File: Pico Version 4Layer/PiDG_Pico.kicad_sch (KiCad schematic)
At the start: 83 parts, among them J1 Conn_02x05_Odd_Even, J10 Trig, J11 Laser Enable, J12 Pixel Reset, J14 Pico Socket A, J15 Pico Socket B, J16 Laser En/PWM Trig/GND, J17 USB-C PD in, J18 Laser 1 mode, J19 Laser 2 mode, J2 Conn_02x05_Odd_Even, J3 Conn_02x05_Odd_Even, J4 Conn_02x05_Odd_Even, J5 Conn_02x05_Odd_Even, J6 Conn_02x05_Odd_Even, J7 Laser 1, J8 Laser 2, U1 74LVC1G04, U10 74AHCT1G08, U11 Raspberry Pi Pico 2 W, U12 74LVC1G17, U13 UCC27524, U14 CH224K, U15 AP63205WU, U16 LM66100, U17 LT3065EDD, U18 TPS3700DDC, U2 SN74LVC04AD, U3 74LVC1G00, U4 SN74LVC04AD, U5 74LVC1G04, U6 SN74LVC04AD, U7 74AHCT1G08, U8 74AHCT1G08, U9 NCP718xSN180

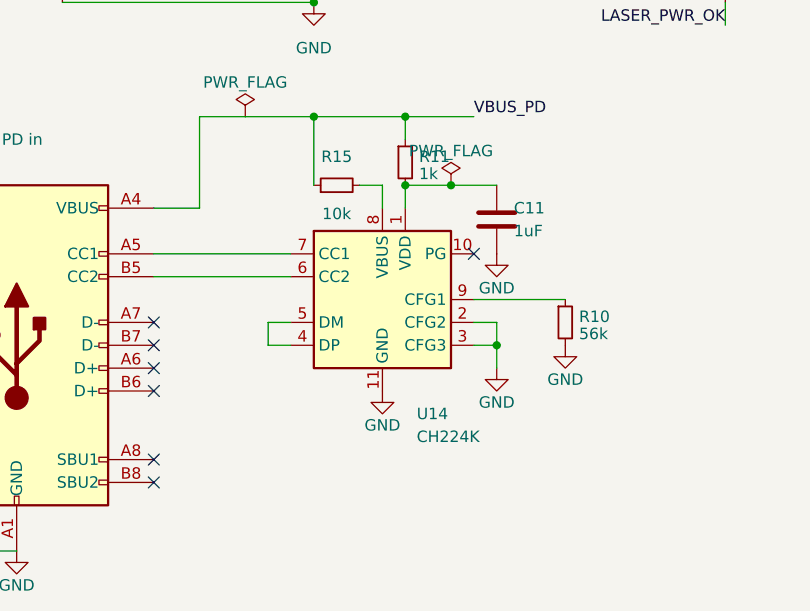
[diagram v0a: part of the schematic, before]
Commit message: Update Pico hardware and fabrication files
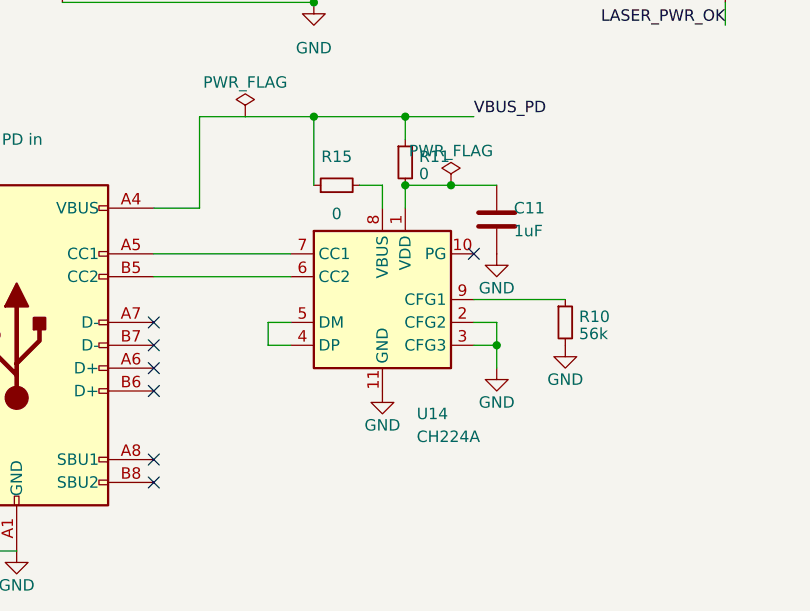
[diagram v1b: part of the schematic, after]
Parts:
- R11: value 1k -> 0
- R15: value 10k -> 0
- U14: value CH224K -> CH224A
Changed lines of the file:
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@@
 			)
 		)
-		(property "Value" "10k"
+		(property "Value" "0"
 			(at 360.68 155.575 90)
 			(show_name no)
@@
 			)
 		)
-		(property "Description" "CH224K VBUS sense resistor (datasheet: 10k)"
+		(property "Description" "CH224A VBUS (pin 8) shorted to VHV: 0 ohm, per WCH guide 7.2.1 (was 10k for CH224K)"
 			(at 360.68 152.4 0)
 			(hide yes)
@@
 			)
 		)
-		(property "Value" "CH224K"
+		(property "Value" "CH224A"
 			(at 369.57 180.34 0)
 			(show_name no)
@@
 			)
 		)
-		(property "Description" "USB PD sink controller. R10 = 56k on CFG1 requests 15 V."
+		(property "Description" "USB PD sink controller, WCH CH224A (pin-compatible successor of the discontinued CH224K). R10 = 56k on CFG1 requests 15 V."
 			(at 365.76 165.1 0)
 			(hide yes)
@@
 			)
 		)
-		(property "Description" "CH224K CFG1: 56k to GND requests 15 V (6k8=9 V, 24k=12 V, open=20 V)"
+		(property "Description" "CH224A CFG1: 56k to GND requests 15 V (6k8=9 V, 24k=12 V, 120k=20 V, 210k=28 V; open is outside the table)"
 			(at 386.08 167.64 0)
 			(hide yes)
@@
 			)
 		)
-		(property "Value" "1k"
+		(property "Value" "0"
 			(at 369.824 151.13 0)
 			(show_name no)
@@
 			)
 		)
-		(property "Description" "CH224K VDD feed (datasheet: 1k). 1206: dissipates 0.14 W at 15 V"
+		(property "Description" "CH224A VHV (pin 1) feed: 0 ohm, per WCH CH224K-to-CH224A guide 7.2.1 (was 1k for CH224K VDD)"
 			(at 368.3 149.86 0)
 			(hide yes)
@@
 			)
 		)
-		(property "Description" "CH224K VDD decoupling"
+		(property "Description" "CH224A VHV decoupling (on VBUS_PD, up to 20 V)"
 			(at 378.46 156.21 0)
 			(hide yes)
